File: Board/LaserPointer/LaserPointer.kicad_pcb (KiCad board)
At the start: 2 copper layers, 47 x 58.4 mm, 21 parts, among them J1 S1, J2 S2, J3 S3, J4 Barrel_Jack, J5 LCD, U1 74HC595

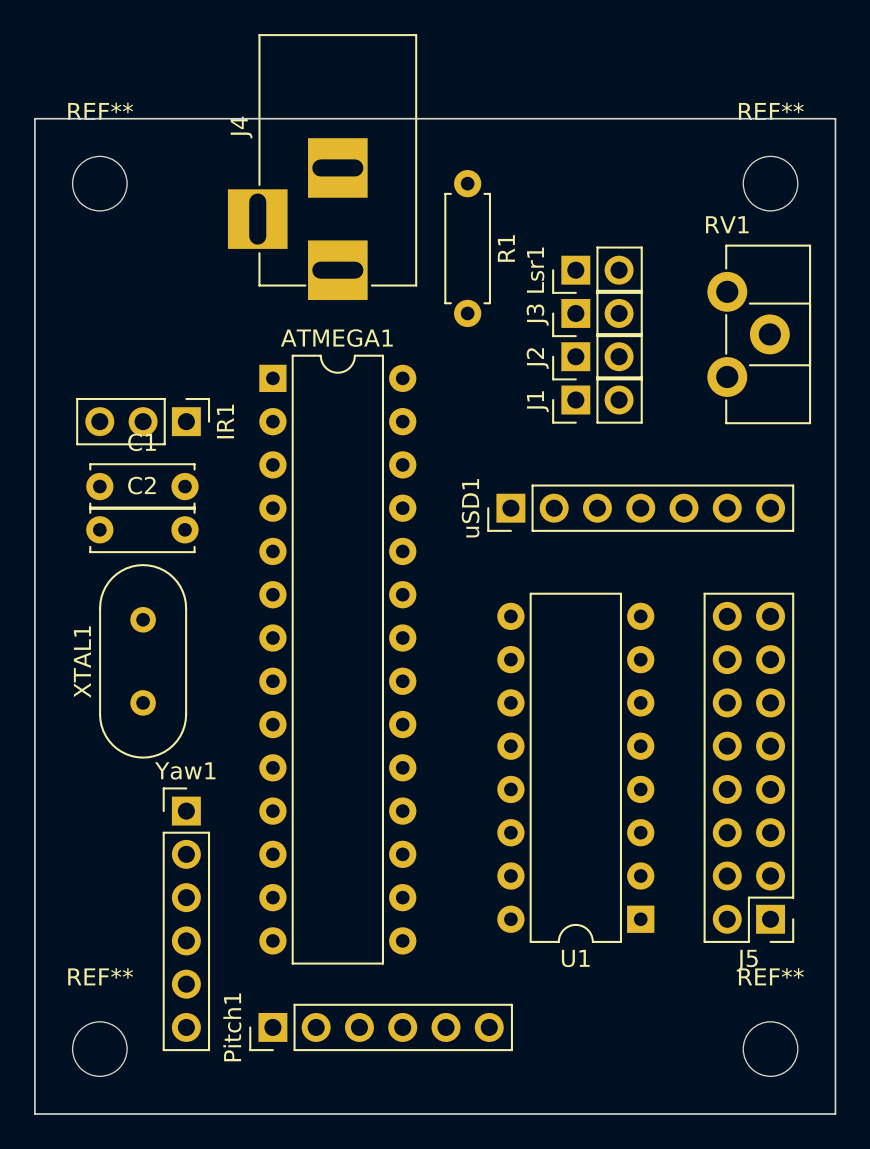
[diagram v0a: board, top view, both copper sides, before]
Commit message: Board updates
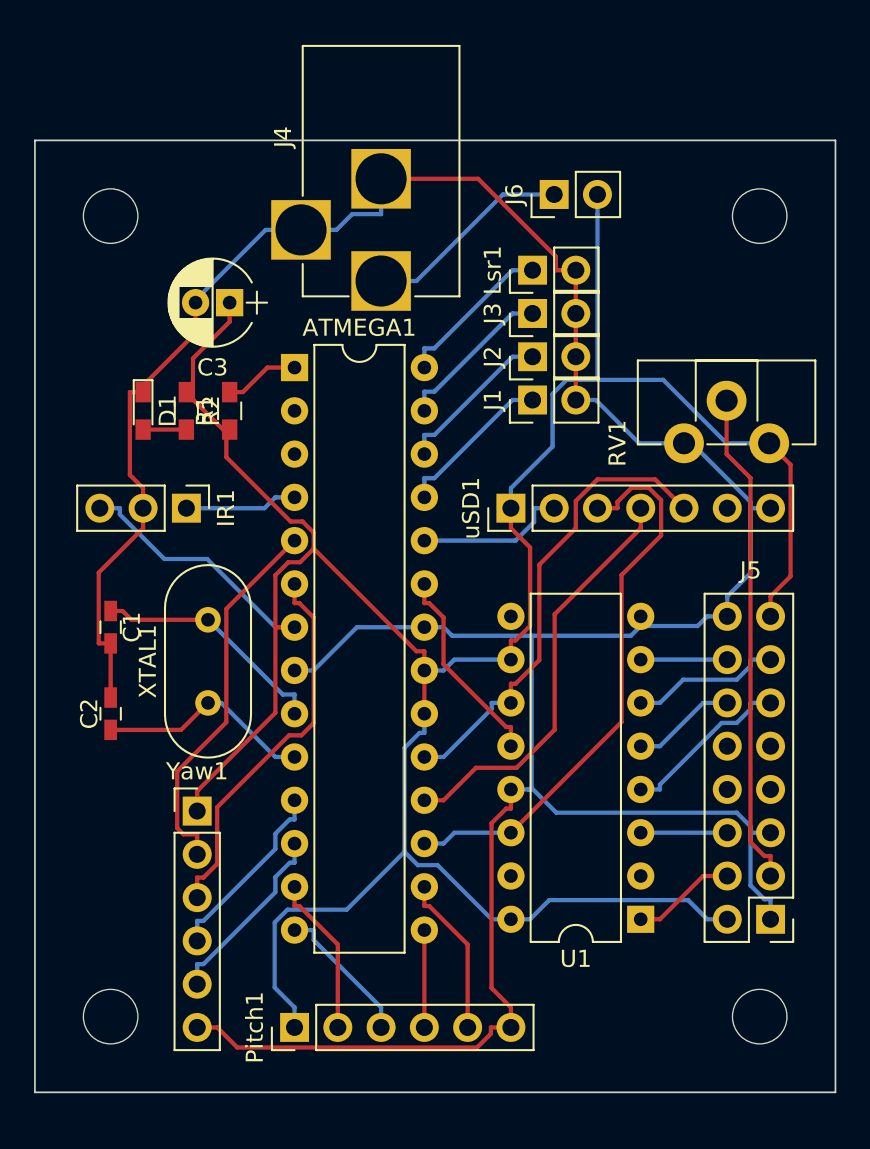
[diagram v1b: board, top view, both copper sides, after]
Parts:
- added C3: CP, Capacitors_THT:CP_Radial_D5.0mm_P2.00mm, F.Cu at (94.0, 81.9)
- added D1: LED, LEDs:LED_0603_HandSoldering, F.Cu at (88.9, 88.3)
- added J6: PWR_SW, Pin_Headers:Pin_Header_Straight_1x02_Pitch2.54mm, F.Cu at (113.0, 75.6)
- added R2: R, Resistors_SMD:R_0603_HandSoldering, F.Cu at (91.4, 88.3)
- C1, C2: footprint Capacitors_THT:C_Disc_D6.0mm_W2.5mm_P5.00mm -> Capacitors_SMD:C_0603_HandSoldering
- R1: footprint Resistors_THT:R_Axial_DIN0207_L6.3mm_D2.5mm_P7.62mm_Horizontal -> Resistors_SMD:R_0603_HandSoldering
- moved R1 19.3 mm to (94.0, 88.3), turned to 90 degrees
- moved C2 10.8 mm to (87.0, 106.0), turned to 90 degrees
- moved RV1 9.25 mm to (120.7, 90.2), turned to 90 degrees
- moved C1 8.28 mm to (87.0, 101.0), turned to 270 degrees
- moved IR1 5.08 mm to (91.4, 94.0)
- moved XTAL1 3.81 mm to (92.7, 105.4)
- moved J4 2.62 mm to (102.9, 80.6)
- moved J1 2.54 mm to (111.8, 87.6)
- moved J2 2.54 mm to (111.8, 85.1)
- moved J3 2.54 mm to (111.8, 82.5)
- moved Lsr1 2.54 mm to (111.8, 80.0)
- moved H3 2.01 mm to (125.1, 123.8)
- moved H4 2.01 mm to (87.0, 123.8)
- moved H1 2.01 mm to (87.0, 76.8)
- moved H2 2.01 mm to (125.1, 76.8)
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- renumbered REF** to H1, REF** to H2, REF** to H3, REF** to H4
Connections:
- J4 pad 1: VCC -> Net-(J4-Pad1)
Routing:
- net GND: track 0.00 -> 179.3 mm
- net VCC: track 0.00 -> 172.3 mm
- net /SPI_MOSI: track 0.00 -> 33.3 mm
- net Net-(J5-Pad3): track 0.00 -> 29.2 mm
- net /SPI_SCK: track 0.00 -> 27.8 mm
- net /SPI_MISO: track 0.00 -> 24.5 mm
- net /Yaw2: track 0.00 -> 22.5 mm
- net /Yaw1: track 0.00 -> 22.2 mm
- net Net-(ATMEGA1-Pad9): track 0.00 -> 14.0 mm
- net Net-(ATMEGA1-Pad10): track 0.00 -> 12.8 mm
- net Net-(J4-Pad1): track 0.00 -> 12.3 mm
- net /LCD_SS: track 0.00 -> 12.0 mm
- net /Yaw4: track 0.00 -> 11.0 mm
- net /Yaw3: track 0.00 -> 11.0 mm
- net /LCD4: track 0.00 -> 10.1 mm
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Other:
- board size 47 x 58.4 mm -> 47 x 55.9 mm
- board text added: "Version 0.1 Feb. 2018"
